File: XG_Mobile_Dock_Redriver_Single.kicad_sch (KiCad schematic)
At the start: 117 parts, among them J1 5-1775443-8, J13 39301240, J14 I2C1, J2 20455-040E-76, J3 20455-040E-76, J4 469911008, J7 10147430-113T0LF, SW1 SW_Push, U1 DS320PR810NJXR, U7 TPS7A8400ARGRR, U8 TPS7A8400ARGRR

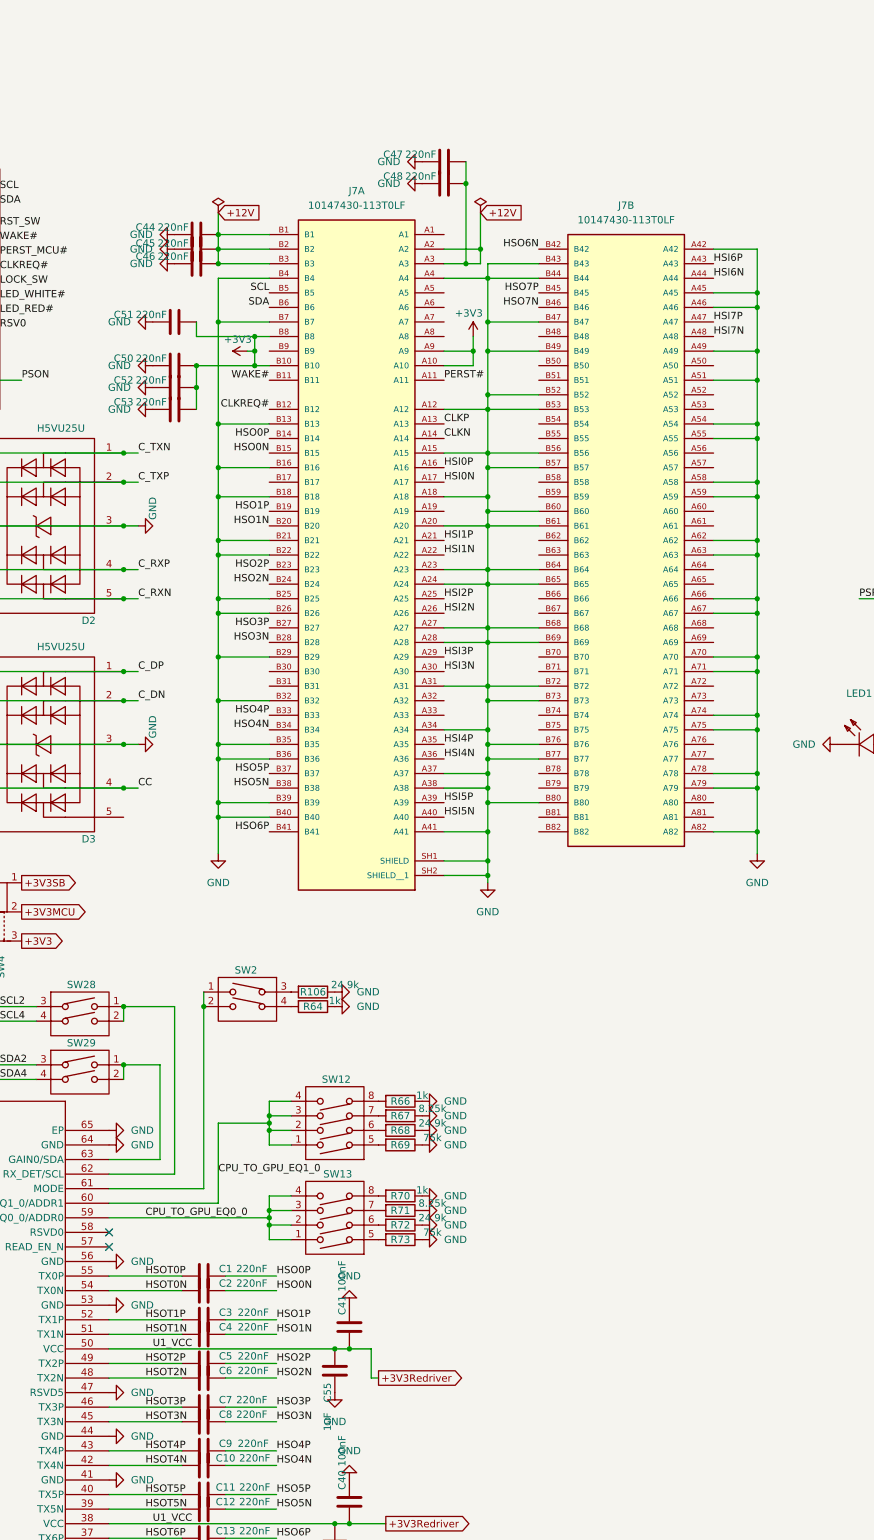
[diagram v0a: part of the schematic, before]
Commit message: new connector
new connector
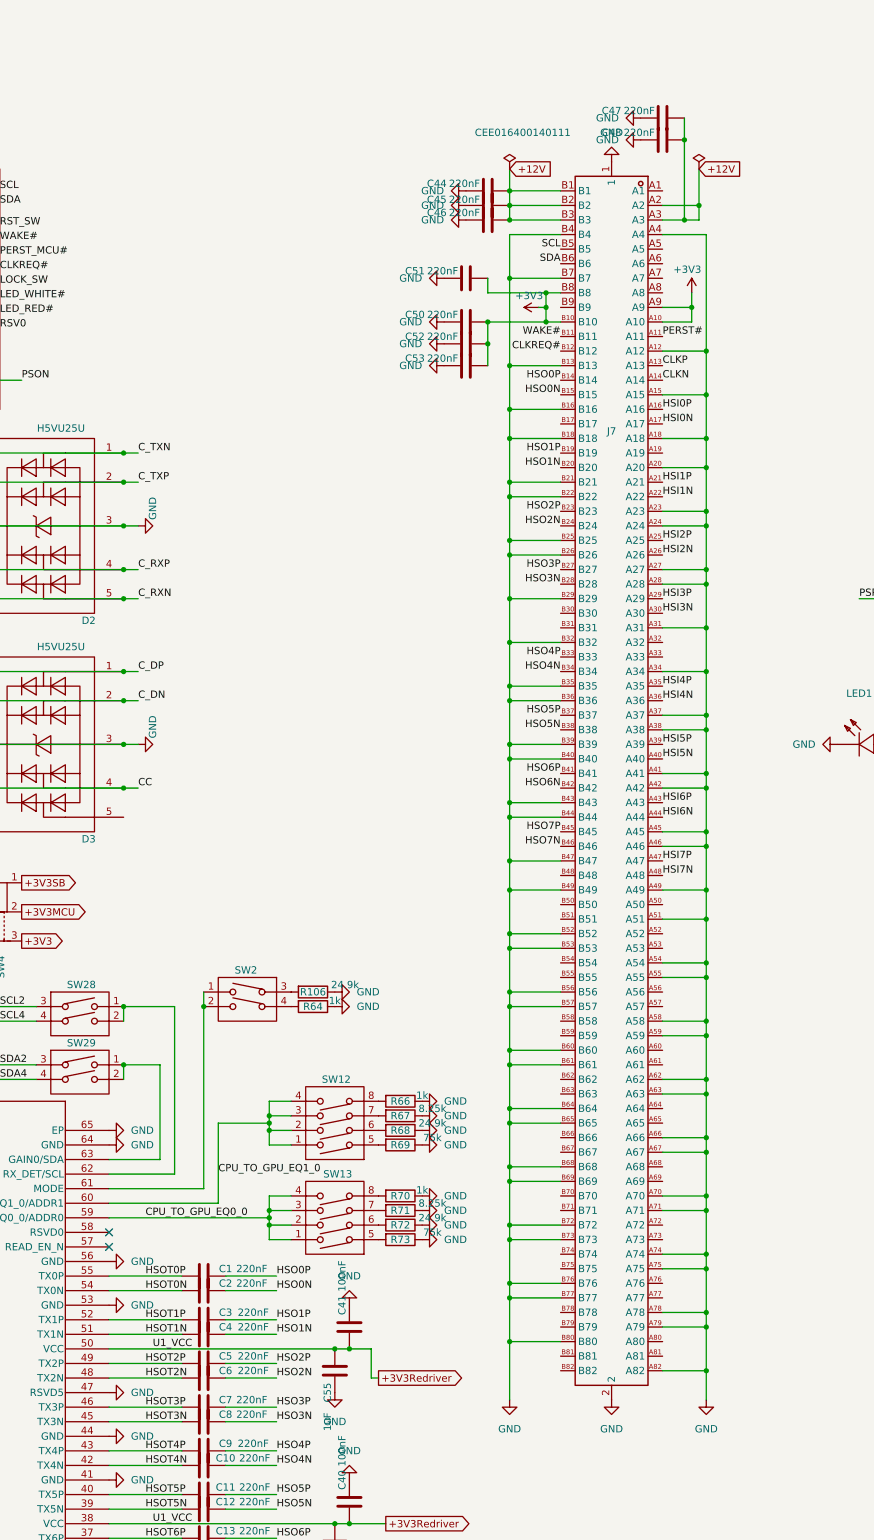
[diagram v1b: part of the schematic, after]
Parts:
- removed unit 2 of J7
- J7: value 10147430-113T0LF -> CEE016400140111; footprint 10147430-113T0LF:AMPHENOL_10147430-113T0LF -> CEE016400140111:CONN-SMD_164P-P1.00-CEE016400140111; symbol 10147430-113T0LF:10147430-113T0LF -> CEE016400140111:CEE016400140111; LCSC C5039496 -> C4762196; LCSC Part Name (none) -> 1mm P数:164P; Manufacturer (none) -> Amphenol; Manufacturer Part (none) -> CEE016400140111; Part_Number 10147430-113T0LF -> CEE016400140111; Supplier (none) -> LCSC; Supplier Part (none) -> C4762196
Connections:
- net GND: now also J7.1, J7.2, J7.A42, J7.A45, J7.A46, J7.A49, J7.A51, J7.A54, J7.A55, J7.A58, J7.A59, J7.A62, J7.A63, J7.A66, J7.A67, J7.A70, J7.A71, J7.A74, J7.A75, J7.A78, J7.A79, J7.A82, J7.B43, J7.B44, J7.B47, J7.B49, J7.B52, J7.B53, J7.B56, J7.B57, J7.B60, J7.B61, J7.B64, J7.B65, J7.B68, J7.B69, J7.B72, J7.B73, J7.B76, J7.B77, J7.B80; no longer J7.SH1 (SHIELD), J7.SH2 (SHIELD__1)
- net HSI6N: now also J7.A44
- net HSI6P: now also J7.A43
- net HSI7N: now also J7.A48
- net HSI7P: now also J7.A47
- net HSO6N: now also J7.B42
- net HSO7N: now also J7.B46
- net HSO7P: now also J7.B45
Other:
- moved on the sheet: C44, C45, C46, C47, C48, C50, C51, C52, C53
